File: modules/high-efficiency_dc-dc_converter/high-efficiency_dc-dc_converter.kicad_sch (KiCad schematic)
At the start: 13 parts, among them U1 ISl91127IR

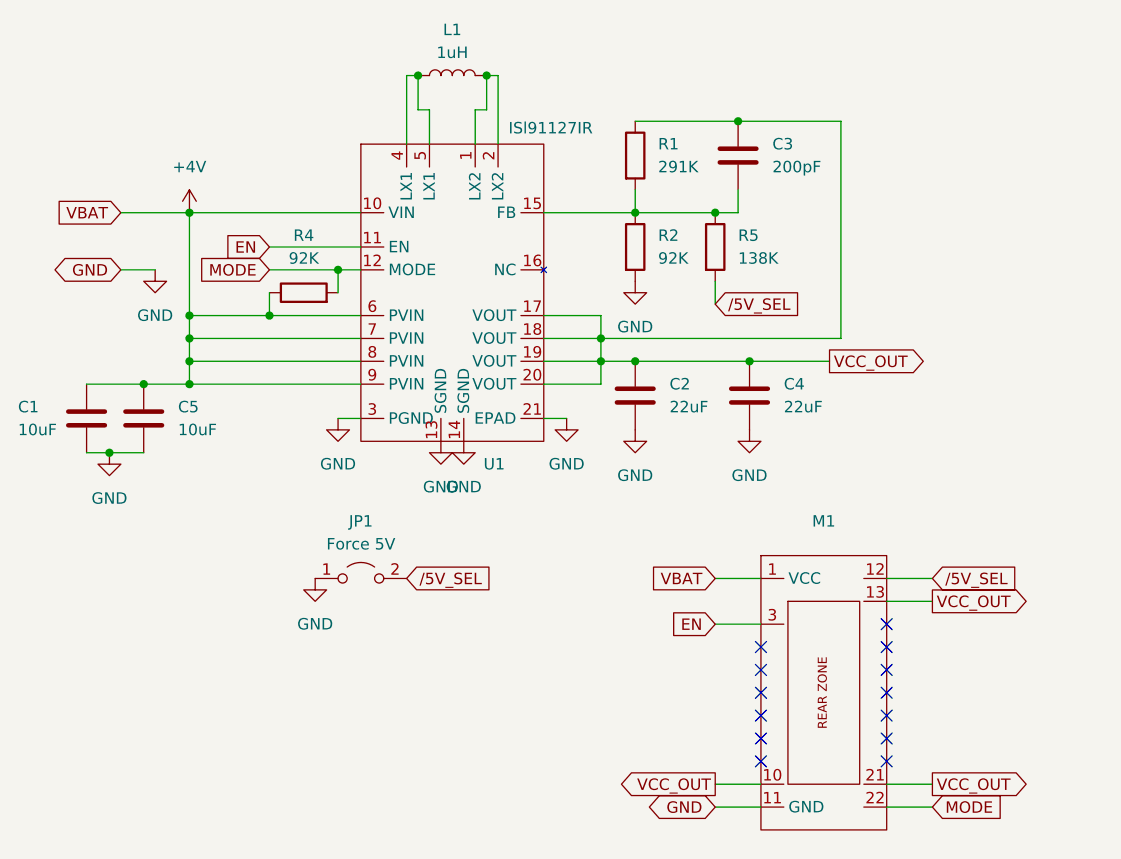
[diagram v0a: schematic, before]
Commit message: Updating all modules
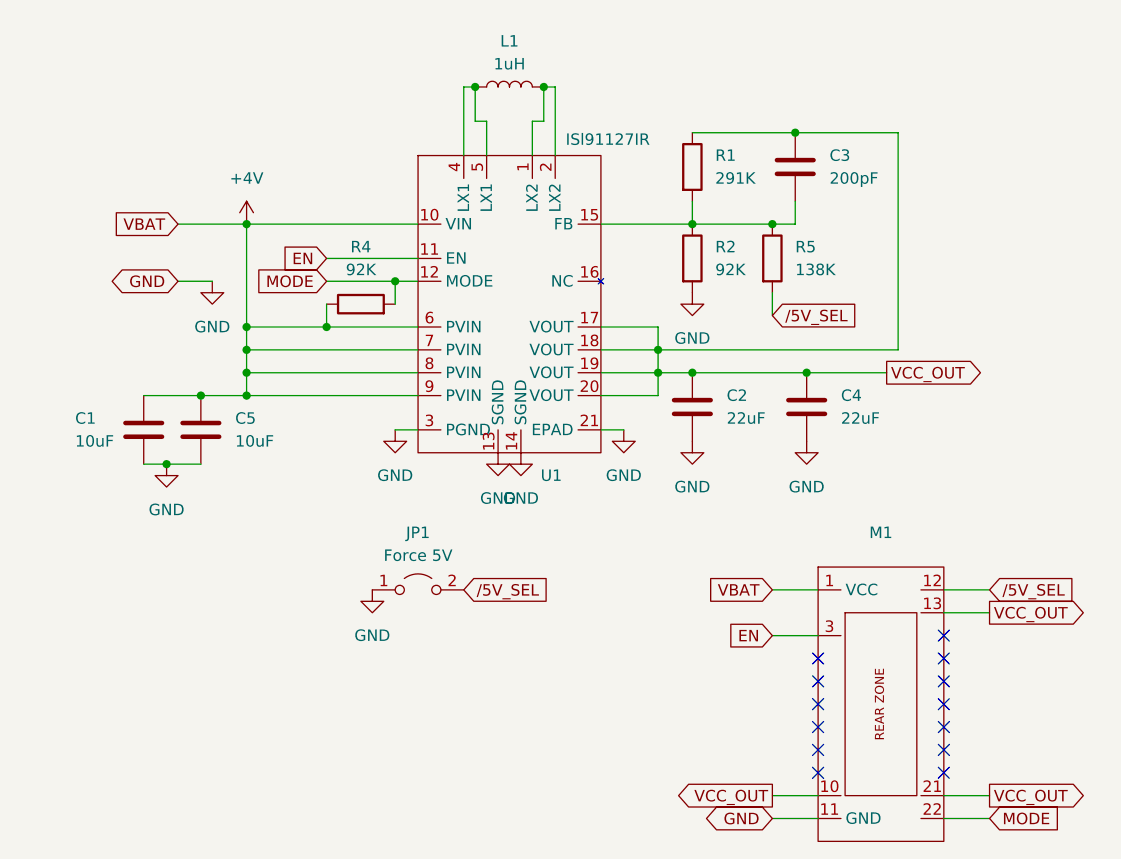
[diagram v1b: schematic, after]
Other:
- moved on the sheet: C1, C2, C3, C4, C5, JP1, L1, M1, R1, R2, R4, R5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
